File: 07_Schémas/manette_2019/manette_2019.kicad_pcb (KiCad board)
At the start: 2 copper layers, 150 x 100 mm, 42 parts, among them J1 Power, J2 Screw_Terminal_01x04, J3 Screw_Terminal_01x04, J4 OLED_Display, SW1 Button_A, SW10 Button_DOWN, SW13 Calib, SW2 Button_B, SW3 Button_X, SW4 Button_Y, SW5 Button_START, SW6 Button_SELECT, SW7 Button_RIGHT, SW8 Button_UP, SW9 Button_LEFT, U1 ESP32, U2 ATmega328-PU, U3 MCP23017, U5 ULN2803A, U6 R-783.3-0.5, U7 R-78E5.0-0.5, U8 PCA9306, Y1 Resonator

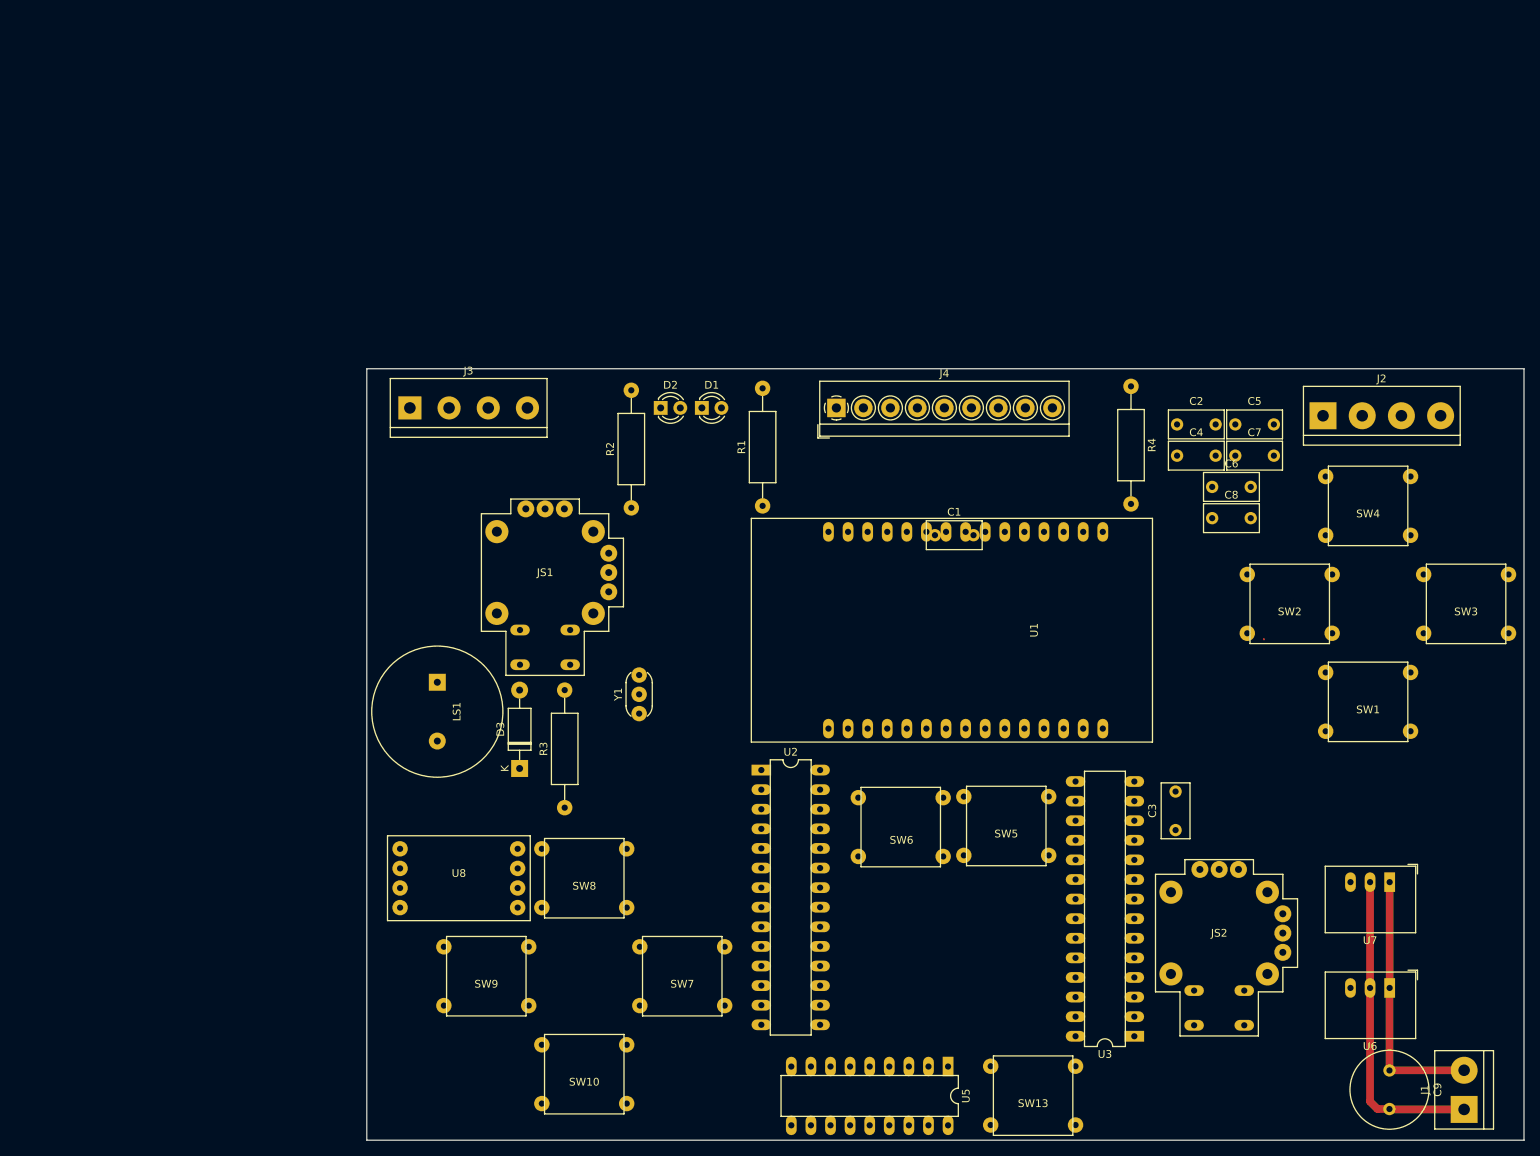
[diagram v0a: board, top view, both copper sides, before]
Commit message: Plans et data movement
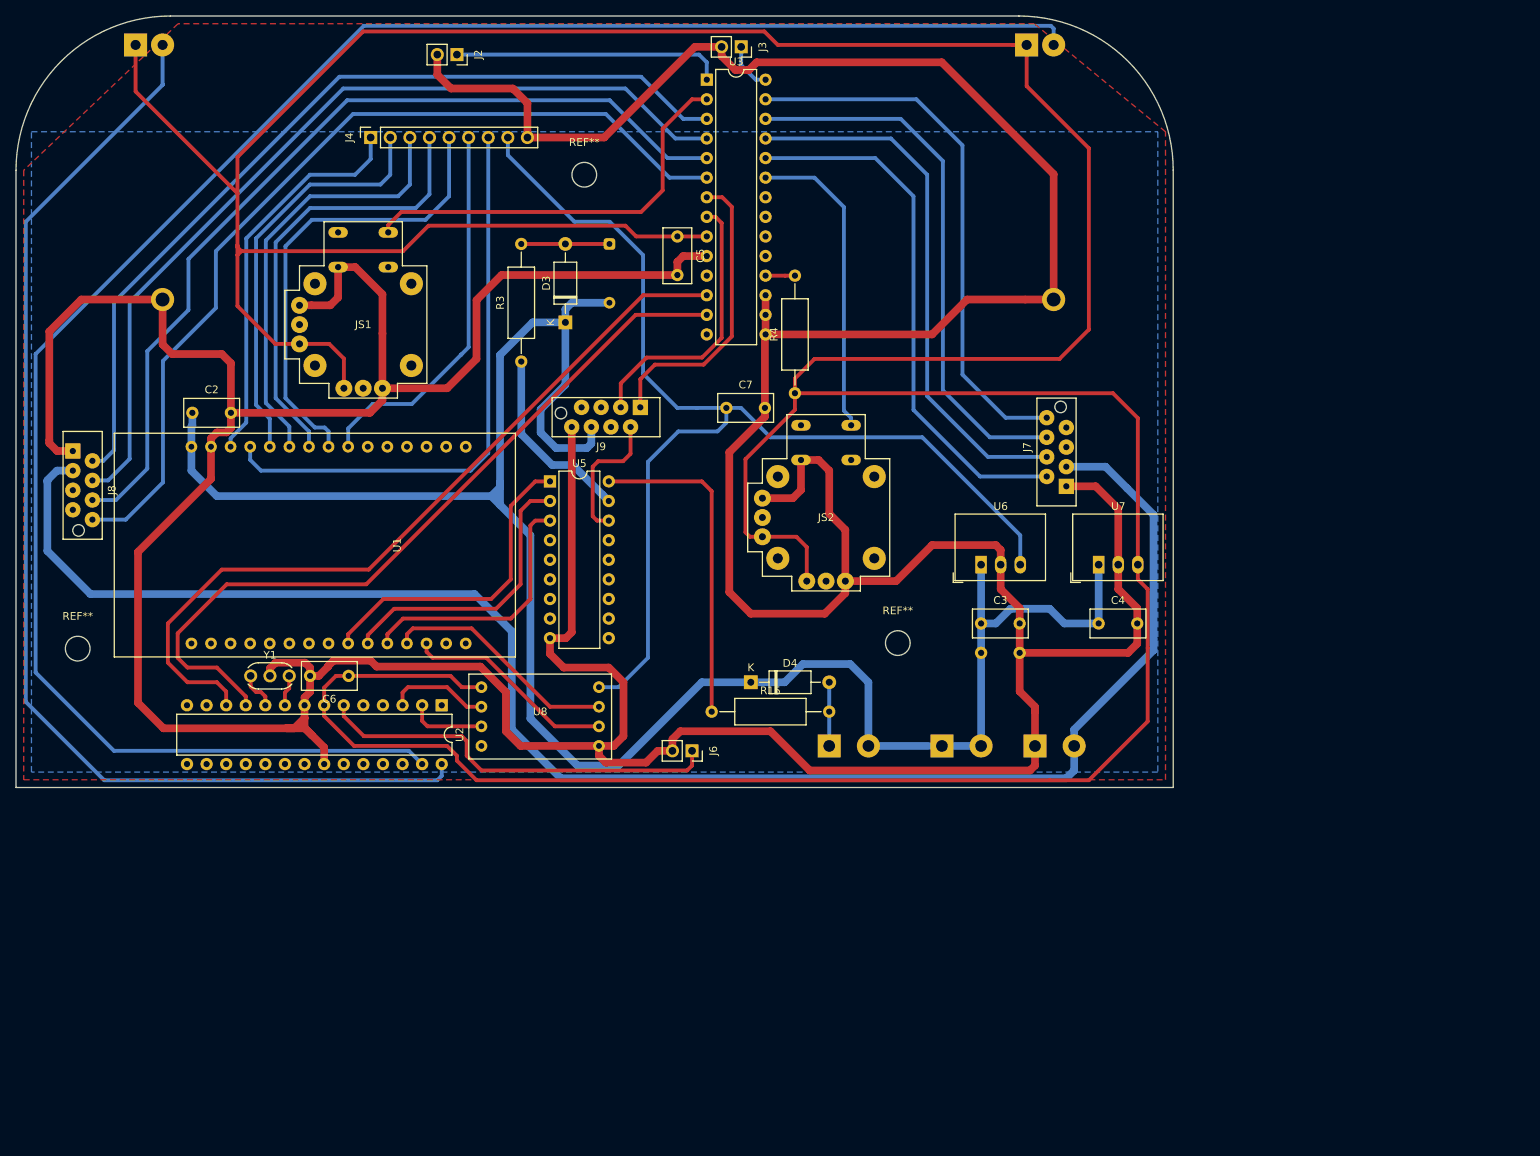
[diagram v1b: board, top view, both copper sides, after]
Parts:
- removed C8: C, Capacitor_THT:C_Rect_L7.0mm_W3.5mm_P5.00mm
- removed C9: C, Capacitor_THT:C_Radial_D10.0mm_H20.0mm_P5.00mm
- removed D1: LED_B, LED_THT:LED_D3.0mm
- removed D2: LED_R, LED_THT:LED_D3.0mm
- removed R1, R2: R, Resistor_THT:R_Axial_DIN0309_L9.0mm_D3.2mm_P15.24mm_Horizontal
- removed SW1: Button_A, Button_Switch_THT:Bouton_MEC
- removed SW10: Button_DOWN, Button_Switch_THT:Bouton_MEC
- removed SW13: Calib, Button_Switch_THT:Bouton_MEC
- removed SW2: Button_B, Button_Switch_THT:Bouton_MEC
- removed SW3: Button_X, Button_Switch_THT:Bouton_MEC
- removed SW4: Button_Y, Button_Switch_THT:Bouton_MEC
- removed SW5: Button_START, Button_Switch_THT:Bouton_MEC
- removed SW6: Button_SELECT, Button_Switch_THT:Bouton_MEC
- removed SW7: Button_RIGHT, Button_Switch_THT:Bouton_MEC
- removed SW8: Button_UP, Button_Switch_THT:Bouton_MEC
- removed SW9: Button_LEFT, Button_Switch_THT:Bouton_MEC
- added D4: D, Diode_THT:D_A-405_P10.16mm_Horizontal, F.Cu at (95.2, 86.4)
- added J10: Alim_LED, TerminalBlock:TerminalBlock_bornier-2_P5.08mm, B.Cu at (132.1, 94.6)
- added J5: Rumble, TerminalBlock:TerminalBlock_bornier-2_P5.08mm, B.Cu at (105.4, 94.6)
- added J6: Calib, Connector_PinSocket_2.54mm:PinSocket_1x02_P2.54mm_Vertical, F.Cu at (87.6, 95.2)
- added J7: Conn_R_Button, manette_2019:Conn_8, F.Cu at (134.9, 55.9)
- added J8: Conn_L_Button, manette_2019:Conn_8, F.Cu at (8.64, 61.5)
- added J9: Conn_Middle_PCB, manette_2019:Conn_8, F.Cu at (75.8, 52.0)
- added R15: R, Resistor_THT:R_Axial_DIN0309_L9.0mm_D3.2mm_P15.24mm_Horizontal, F.Cu at (90.2, 90.2)
- added REF**: MountingHole_3.2mm_M3, MountingHole:MountingHole_3.2mm_M3, F.Cu at (8.00, 82.0)
- added REF**: MountingHole_3.2mm_M3, MountingHole:MountingHole_3.2mm_M3, F.Cu at (114.3, 81.3)
- added REF**: MountingHole_3.2mm_M3, MountingHole:MountingHole_3.2mm_M3, F.Cu at (73.7, 20.6)
- added RV1: R_POT, Potentiometer_THT:Potentiometer_Bourns_PTA2043_Single_Slide, B.Cu at (15.5, 3.75)
- added RV2: R_POT, Potentiometer_THT:Potentiometer_Bourns_PTA2043_Single_Slide, B.Cu at (131.0, 3.75)
- C1: footprint Capacitor_THT:C_Rect_L7.0mm_W3.5mm_P5.00mm -> Capacitor_THT:C_Radial_D10.0mm_H20.0mm_P5.00mm; moved to B.Cu
- J1: value Power -> Vcc; moved to B.Cu
- J2: value Screw_Terminal_01x04 -> L_Bumper; footprint TerminalBlock:TerminalBlock_bornier-4_P5.08mm -> Connector_PinSocket_2.54mm:PinSocket_1x02_P2.54mm_Vertical
- J3: value Screw_Terminal_01x04 -> R_Bumper; footprint TerminalBlock:TerminalBlock_bornier-4_P5.08mm -> Connector_PinSocket_2.54mm:PinSocket_1x02_P2.54mm_Vertical
- J4: footprint TerminalBlock_4Ucon:TerminalBlock_4Ucon_1x09_P3.50mm_Horizontal -> Connector_PinSocket_2.54mm:PinSocket_1x09_P2.54mm_Vertical
- LS1: moved to B.Cu
- U1: footprint ESP32:ESP32 -> manette_2019:ESP32
- U8: footprint PCA9306:PCA9306 -> manette_2019:PCA9306
- moved U3 135.8 mm to (89.5, 8.26), turned to 0 degrees
- moved C2 127.6 mm to (22.9, 51.4)
- moved J2 121.6 mm to (57.1, 5.00), turned to 270 degrees
- moved C6 114.6 mm to (43.1, 85.5), turned to 180 degrees
- moved U5 91.7 mm to (69.2, 60.3), turned to 0 degrees
- moved U1 83.3 mm to (38.7, 68.6)
- moved J1 82.5 mm to (120.0, 94.6), turned to 0 degrees
- moved C5 76.3 mm to (85.7, 28.6), turned to 270 degrees
- moved U6 76.3 mm to (125.1, 71.1), turned to 0 degrees
- moved JS2 74.2 mm to (105.0, 65.0), turned to 180 degrees
- moved J4 69.8 mm to (46.0, 15.7), turned to 90 degrees
- moved C7 66.3 mm to (92.1, 50.8)
- moved J3 63.5 mm to (94.0, 4.00), turned to 270 degrees
- moved LS1 61.0 mm to (76.9, 33.4)
- moved D3 58.1 mm to (71.2, 39.7)
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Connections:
- C2 pad 1: +5V -> VCC
- C3 pad 1: +5V -> VCC
- C4 pad 1: +5V -> VCC
- C6 pad 1: +3.3V -> +5V
- C7 pad 1: VCC -> +3.3V
- D3 pad 1: +3.3V -> VCC
- J1 pad 1: GND -> VCC
- J2 pad 1: Right_trigger -> L_Bumper
- J2 pad 2: R_Bumper -> GND
- J3 pad 1: Left_trigger -> R_Bumper
- J3 pad 2: L_Bumper -> GND
- LS1 pad 2: +3.3V -> VCC
- U1 pad 10: OLEDCS -> DC
- U1 pad 15: Net-(U1-Pad15) -> VCC
- U1 pad 24: Connected -> Rumble
- U1 pad 25: Power -> Buzzer
- U1 pad 26: Buzzer -> Connected
- U1 pad 8: RESET -> OLEDCS
- U1 pad 9: DC -> RESET
- U3 pad 1: Net-(U3-Pad1) -> L_Bumper
- U3 pad 2: Net-(U3-Pad2) -> Left_joystick_button
- U3 pad 21: Button_SELECT -> Net-(U3-Pad21)
- U3 pad 22: Button_START -> Net-(U3-Pad22)
- U3 pad 23: L_Bumper -> Right_joystick_button
- U3 pad 24: R_Bumper -> Button_A
- U3 pad 25: Button_X -> Button_B
- U3 pad 27: Button_B -> Button_X
- U3 pad 28: Button_A -> R_Bumper
- U3 pad 3: R_joystick_button -> Button_DOWN
- U3 pad 4: L_joystick_button -> Button_RIGHT
- U3 pad 5: Button_LEFT -> Button_UP
- U3 pad 6: Button_UP -> Button_LEFT
- U3 pad 7: Button_RIGHT -> Button_SELECT
- U3 pad 8: Button_DOWN -> Button_START
- U5 pad 1: Connected -> Rumble
- U5 pad 16: Net-(R3-Pad1) -> Conn_LED_On
- U5 pad 17: Net-(R2-Pad1) -> Net-(R3-Pad1)
- U5 pad 2: Power -> Buzzer
- U5 pad 3: Buzzer -> Connected
- U8 pad 2: RX_Atmega -> TX_Atmega
- U8 pad 3: TX_Atmega -> RX_Atmega
- U8 pad 6: RX_ESP32 -> TX_ESP32
- U8 pad 7: TX_ESP32 -> RX_ESP32
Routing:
- net GND: track 41.1 -> 754.7 mm
- net +5V: track 0.00 -> 579.6 mm
- net R_trigger: track 0.00 -> 248.1 mm
- net VCC: track 34.1 -> 267.3 mm
- net VCC_LED: track 0.00 -> 217.8 mm
- net L_trigger: track 0.00 -> 152.4 mm
- net +3.3V: track 0.00 -> 149.4 mm
- net Button_LEFT: track 0.00 -> 118.4 mm
- net Button_UP: track 0.00 -> 117.0 mm
- net Button_RIGHT: track 0.00 -> 115.3 mm
- net Button_DOWN: track 0.00 -> 113.8 mm
- net SCL: track 0.00 -> 103.4 mm
- net SDA: track 0.00 -> 100.9 mm
- net MISO: track 0.00 -> 75.0 mm
- net Button_Y: track 0.00 -> 71.0 mm
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- added copper zone on F.Cu, net GND
- added copper zone on B.Cu, net VCC
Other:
- outline, holes or cut-outs redrawn
- net class Default: trace_width 0.25 -> 0.5
